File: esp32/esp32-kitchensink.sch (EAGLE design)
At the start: 202 parts, among them J14 MEM2075-00-140-01-A, J16 10103592-0001LF-EK, J19 PJ-102AH, Q1 MMBT3904_R1, Q2 MMBT3904_R1, Q3 AO3401, Q4 PN2222A-SOT-23, Q5 IRF7341TRPBF, U1 ESP32-WROOM-32D, U10 AH1807-W-7SC59_DIO-M, U11 DS3231M+TRL21-0042B_16_MXM-M, U12 MC74HC595ADR2GSOIC-16_ONS-M, U2 AP2111H-3.3TRG1SOT-223_DIO-M, U3 CP2102N-A02-GQFN24QFN24_CP210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, U4 MCP73831T-3ACI/OTSOT-23-5_MC_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, U5 TPS613222ADBVTDBV0005A_M, U6 PAM2401SCADJ, U7 ZXBM5210-SP-13SOIC8_ZXBM5210-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, U8 BSS138SOT-23_3L_ONS-M, U9 TS2940CW50_RPG, X1 TMP235_DCKR

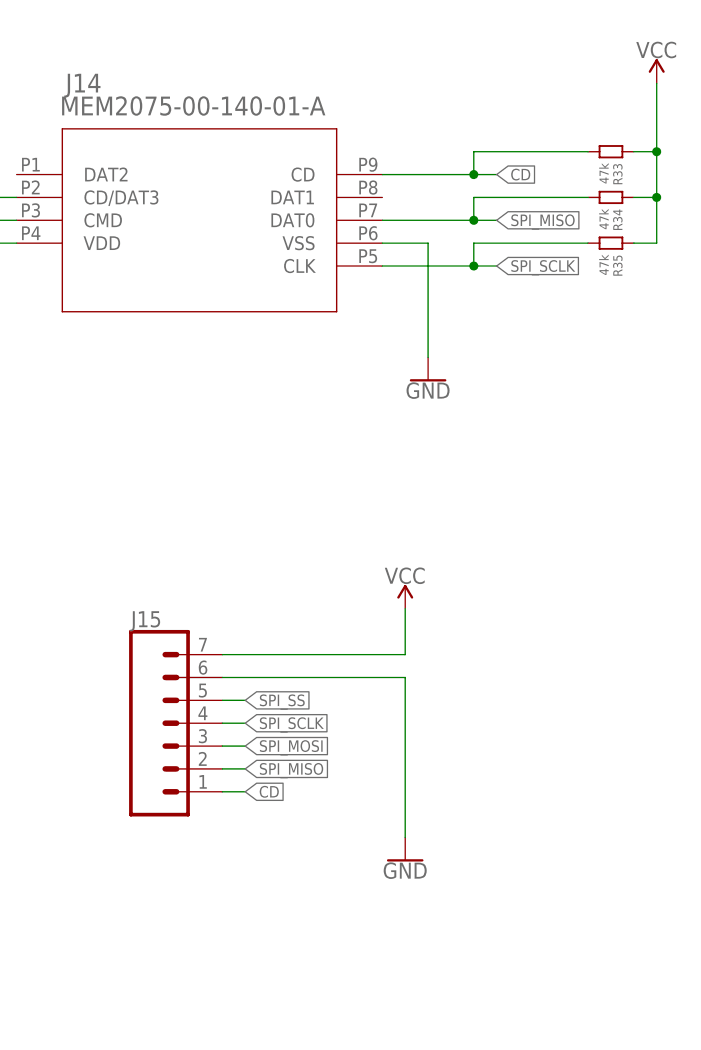
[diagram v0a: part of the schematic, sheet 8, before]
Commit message: Updates to larger kitchen sink files
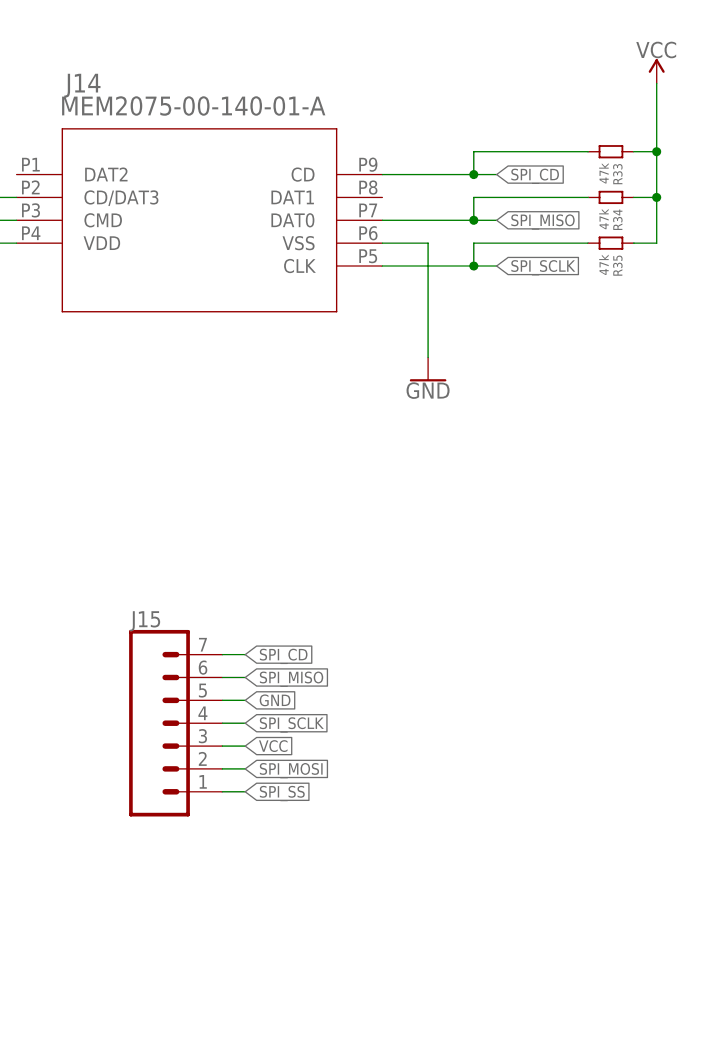
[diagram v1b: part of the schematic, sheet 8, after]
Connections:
- removed net CD: J14.CD, J15.1, R33.2
- new net SPI_CD: J14.CD, J15.7, R33.2
- net GND: now also J15.5; no longer J15.6
- net SPI_MISO: now also J15.6; no longer J15.2
- net SPI_MOSI: now also J15.2; no longer J15.3
- net SPI_SS: now also J15.1; no longer J15.5
- net VCC: now also J15.3; no longer J15.7
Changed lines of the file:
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@@
 <part name="SUPPLY22" library="SparkFun-PowerSymbols" library_urn="urn:adsk.eagle:library:530" deviceset="VCC" device=""/>
 <part name="J15" library="SparkFun-Connectors" library_urn="urn:adsk.eagle:library:513" deviceset="CONN_07" device="LONGPADS" package3d_urn="urn:adsk.eagle:package:38135/1"/>
-<part name="GND52" library="SparkFun-PowerSymbols" library_urn="urn:adsk.eagle:library:530" deviceset="GND" device=""/>
-<part name="SUPPLY20" library="SparkFun-PowerSymbols" library_urn="urn:adsk.eagle:library:530" deviceset="VCC" device=""/>
 <part name="J16" library="UltraLibrarianParts" deviceset="10103592-0001LF-EK" device=""/>
 <part name="J3" library="SparkFun-Connectors" library_urn="urn:adsk.eagle:library:513" deviceset="CONN_03" device="LONGPADS" package3d_urn="urn:adsk.eagle:package:38068/1"/>
@@
 <attribute name="NAME" x="177.8" y="79.248" size="1.778" layer="95" font="vector"/>
 </instance>
-<instance part="GND52" gate="1" x="208.28" y="53.34" smashed="yes">
-<attribute name="VALUE" x="208.28" y="53.086" size="1.778" layer="96" align="top-center"/>
-</instance>
-<instance part="SUPPLY20" gate="G$1" x="208.28" y="81.28" smashed="yes">
-<attribute name="VALUE" x="208.28" y="84.074" size="1.778" layer="96" align="bottom-center"/>
-</instance>
 </instances>
 <busses>
@@
 </segment>
 <segment>
-<pinref part="J15" gate="G$1" pin="6"/>
-<wire x1="187.96" y1="73.66" x2="208.28" y2="73.66" width="0.1524" layer="91"/>
-<wire x1="208.28" y1="73.66" x2="208.28" y2="55.88" width="0.1524" layer="91"/>
-<pinref part="GND52" gate="1" pin="GND"/>
+<pinref part="J15" gate="G$1" pin="5"/>
+<wire x1="187.96" y1="71.12" x2="190.5" y2="71.12" width="0.1524" layer="91"/>
+<label x="190.5" y="71.12" size="1.27" layer="95" xref="yes"/>
 </segment>
 </net>
@@
 </segment>
 <segment>
-<pinref part="J15" gate="G$1" pin="7"/>
-<wire x1="187.96" y1="76.2" x2="208.28" y2="76.2" width="0.1524" layer="91"/>
-<wire x1="208.28" y1="76.2" x2="208.28" y2="81.28" width="0.1524" layer="91"/>
-<pinref part="SUPPLY20" gate="G$1" pin="VCC"/>
+<pinref part="J15" gate="G$1" pin="3"/>
+<wire x1="187.96" y1="66.04" x2="190.5" y2="66.04" width="0.1524" layer="91"/>
+<label x="190.5" y="66.04" size="1.27" layer="95" xref="yes"/>
 </segment>
 </net>
@@
 </segment>
 <segment>
-<pinref part="J15" gate="G$1" pin="2"/>
-<wire x1="187.96" y1="63.5" x2="190.5" y2="63.5" width="0.1524" layer="91"/>
-<label x="190.5" y="63.5" size="1.27" layer="95" xref="yes"/>
+<pinref part="J15" gate="G$1" pin="6"/>
+<wire x1="187.96" y1="73.66" x2="190.5" y2="73.66" width="0.1524" layer="91"/>
+<label x="190.5" y="73.66" size="1.27" layer="95" xref="yes"/>
 </segment>
 </net>
@@
 </segment>
 <segment>
-<pinref part="J15" gate="G$1" pin="3"/>
-<wire x1="187.96" y1="66.04" x2="190.5" y2="66.04" width="0.1524" layer="91"/>
-<label x="190.5" y="66.04" size="1.27" layer="95" xref="yes"/>
+<pinref part="J15" gate="G$1" pin="2"/>
+<wire x1="187.96" y1="63.5" x2="190.5" y2="63.5" width="0.1524" layer="91"/>
+<label x="190.5" y="63.5" size="1.27" layer="95" xref="yes"/>
 </segment>
 </net>
@@
 </segment>
 <segment>
-<pinref part="J15" gate="G$1" pin="5"/>
-<wire x1="187.96" y1="71.12" x2="190.5" y2="71.12" width="0.1524" layer="91"/>
-<label x="190.5" y="71.12" size="1.27" layer="95" xref="yes"/>
+<pinref part="J15" gate="G$1" pin="1"/>
+<wire x1="187.96" y1="60.96" x2="190.5" y2="60.96" width="0.1524" layer="91"/>
+<label x="190.5" y="60.96" size="1.27" layer="95" xref="yes"/>
 </segment>
 </net>
@@
 </segment>
 </net>
-<net name="CD" class="0">
-<segment>
-<pinref part="J14" gate="A" pin="CD"/>
-<wire x1="205.74" y1="129.54" x2="215.9" y2="129.54" width="0.1524" layer="91"/>
-<label x="218.44" y="129.54" size="1.27" layer="95" xref="yes"/>
-<wire x1="215.9" y1="129.54" x2="218.44" y2="129.54" width="0.1524" layer="91"/>
-<wire x1="215.9" y1="129.54" x2="215.9" y2="132.08" width="0.1524" layer="91"/>
-<junction x="215.9" y="129.54"/>
-<wire x1="215.9" y1="132.08" x2="228.6" y2="132.08" width="0.1524" layer="91"/>
-<pinref part="R33" gate="G$1" pin="2"/>
-</segment>
-<segment>
-<pinref part="J15" gate="G$1" pin="1"/>
-<wire x1="187.96" y1="60.96" x2="190.5" y2="60.96" width="0.1524" layer="91"/>
-<label x="190.5" y="60.96" size="1.27" layer="95" xref="yes"/>
-</segment>
-</net>
 <net name="I2C_SCL" class="0">
 <segment>
@@
 </segment>
 </net>
+<net name="SPI_CD" class="0">
+<segment>
+<pinref part="J14" gate="A" pin="CD"/>
+<wire x1="205.74" y1="129.54" x2="215.9" y2="129.54" width="0.1524" layer="91"/>
+<label x="218.44" y="129.54" size="1.27" layer="95" xref="yes"/>
+<wire x1="215.9" y1="129.54" x2="218.44" y2="129.54" width="0.1524" layer="91"/>
+<wire x1="215.9" y1="129.54" x2="215.9" y2="132.08" width="0.1524" layer="91"/>
+<junction x="215.9" y="129.54"/>
+<wire x1="215.9" y1="132.08" x2="228.6" y2="132.08" width="0.1524" layer="91"/>
+<pinref part="R33" gate="G$1" pin="2"/>
+</segment>
+<segment>
+<pinref part="J15" gate="G$1" pin="7"/>
+<wire x1="187.96" y1="76.2" x2="190.5" y2="76.2" width="0.1524" layer="91"/>
+<label x="190.5" y="76.2" size="1.27" layer="95" xref="yes"/>
+</segment>
+</net>
